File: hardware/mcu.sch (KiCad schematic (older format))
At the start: 17 parts, among them U1 TPD4E001-Q1, U2 TPD4E001-Q1, U3 ATmega2561-16AU, U6 TPD4E001-Q1, Y1 CSTCE16M0V53-R0

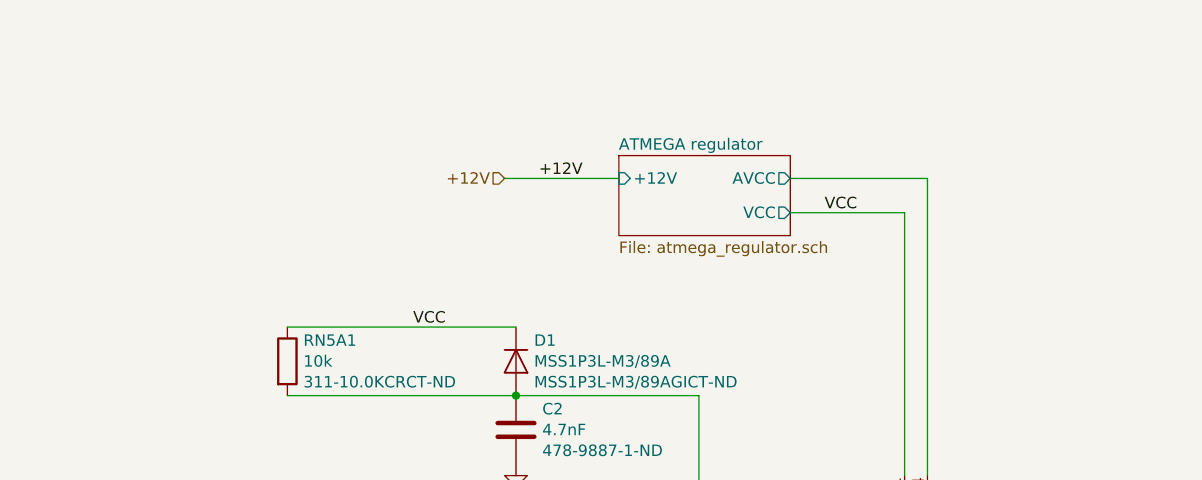
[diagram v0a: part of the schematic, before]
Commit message: rev 2 work in progress
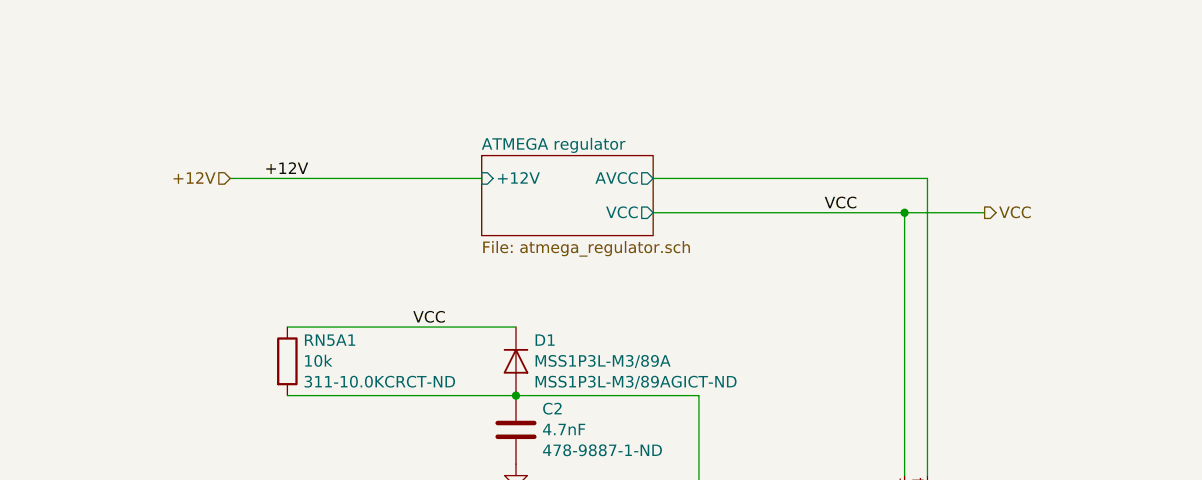
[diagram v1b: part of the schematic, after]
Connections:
- wire segments 103 -> 104
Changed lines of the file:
@@
 $Descr A4 11693 8268
 encoding utf-8
-Sheet 20 23
+Sheet 19 22
 Title ""
 Date ""
@@
 $EndSheet
 $Sheet
-S 5050 1300 750  350
+S 4450 1300 750  350
 U 5D1A080F
 F0 "ATMEGA regulator" 50
 F1 "atmega_regulator.sch" 50
-F2 "+12V" I L 5050 1400 50
-F3 "VCC" O R 5800 1550 50
-F4 "AVCC" O R 5800 1400 50
+F2 "+12V" I L 4450 1400 50
+F3 "VCC" O R 5200 1550 50
+F4 "AVCC" O R 5200 1400 50
 $EndSheet
 Wire Wire Line
-	5800 1550 6300 1550
-Wire Wire Line
 	6300 1550 6300 2700
-Wire Wire Line
-	5800 1400 6400 1400
 Wire Wire Line
 	6400 1400 6400 2700
@@
 Text Label 11850 6300 2    50   ~ 0
 VCC
-Text HLabel 4550 1400 0    50   Input ~ 0
+Text HLabel 3350 1400 0    50   Input ~ 0
 +12V
-Wire Wire Line
-	4550 1400 5050 1400
-Text Label 4700 1400 0    50   ~ 0
+Text Label 3500 1400 0    50   ~ 0
 +12V
 Text Label 11850 6700 2    50   ~ 0
@@
 Wire Wire Line
 	11450 6700 11850 6700
+Wire Wire Line
+	5200 1550 6300 1550
+Wire Wire Line
+	5200 1400 6400 1400
+Wire Wire Line
+	3350 1400 4450 1400
+Text HLabel 6650 1550 2    50   Output ~ 0
+VCC
+Wire Wire Line
+	6300 1550 6650 1550
+Connection ~ 6300 1550
 $EndSCHEMATC
